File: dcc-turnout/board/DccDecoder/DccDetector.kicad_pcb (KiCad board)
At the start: 2 copper layers, 60 x 52 mm, 45 parts, among them J1 Conn_01x02, J2 Conn_01x02, J3 Conn_01x03, J4 Conn_01x02, J5 Conn_01x02, J6 Conn_01x02, J7 Conn_01x04, Q1 BC560, Q2 BC807, Q3 BC817, Q4 NXV90EPR, U1 AMS1117-5.0, U2 6N137S1, U3 PC817, U4 AMS1117-3.3

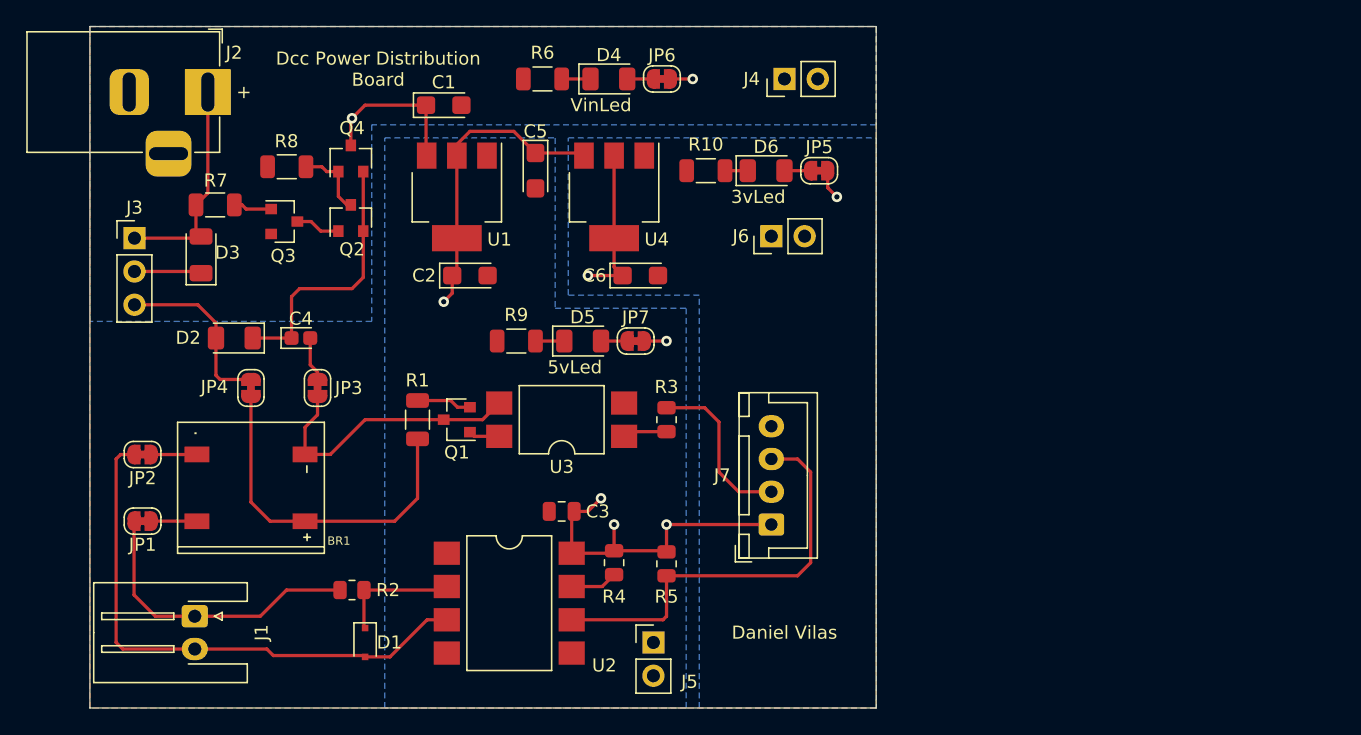
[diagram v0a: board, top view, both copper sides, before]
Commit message: Buck Design
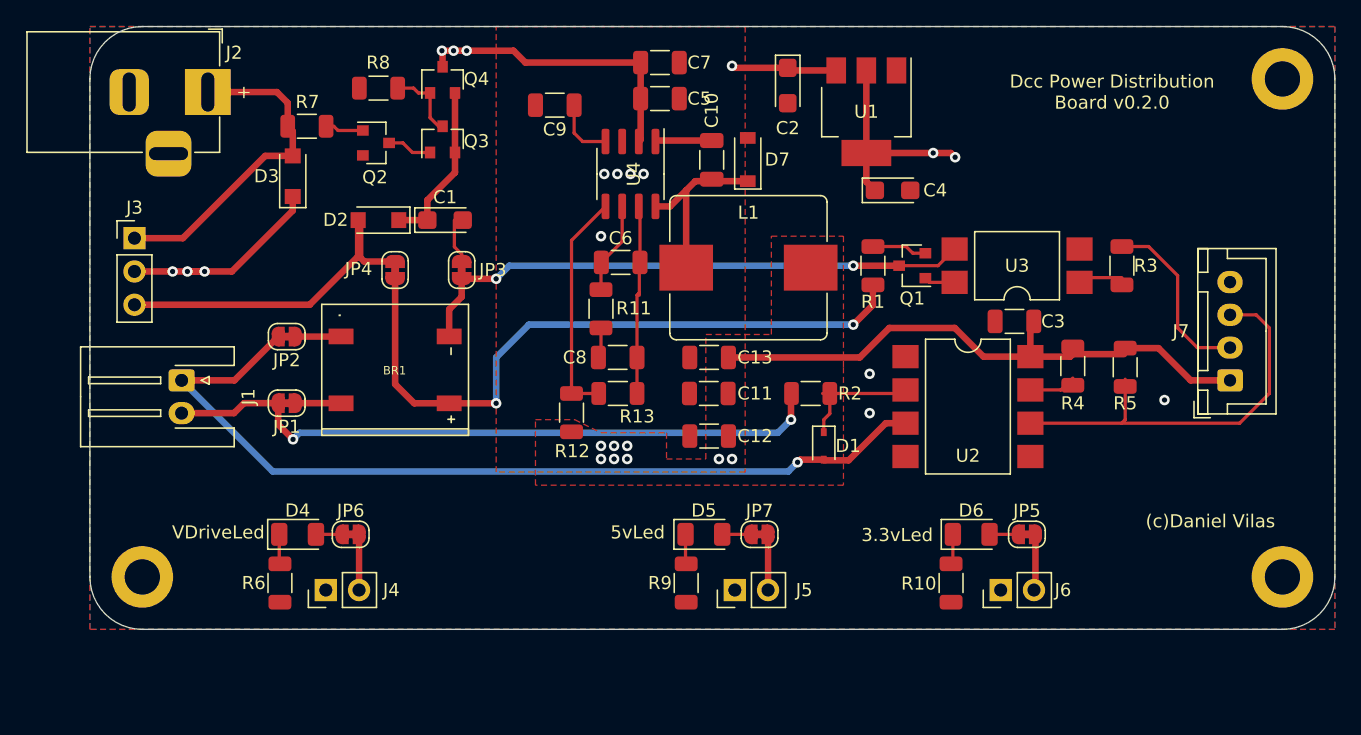
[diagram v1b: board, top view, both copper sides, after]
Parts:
- removed the C1 at (47.0, 26.0)
- removed the C2 at (49.0, 39.0)
- removed the U1 at (48.0, 33.0)
- added C10: 100nf 1m, Capacitor_SMD:C_1206_3216Metric, F.Cu at (67.5, 30.2)
- added C11: 10uf 2m, Capacitor_SMD:C_1206_3216Metric, F.Cu at (67.2, 48.0)
- added C12: 10uf 2m, Capacitor_SMD:C_1206_3216Metric, F.Cu at (67.2, 51.2)
- added C13: 10uf 2m, Capacitor_SMD:C_1206_3216Metric, F.Cu at (67.2, 45.2)
- added C5: 10uf 2m, Capacitor_SMD:C_1206_3216Metric, F.Cu at (63.5, 25.5)
- added C6: 10pf, Capacitor_SMD:C_1206_3216Metric, F.Cu at (60.5, 38.0)
- added C7: 10uf 2m, Capacitor_SMD:C_1206_3216Metric, F.Cu at (63.5, 22.8)
- added C8: 5.6nf, Capacitor_SMD:C_1206_3216Metric, F.Cu at (60.3, 45.2)
- added C9: 8.2nf, Capacitor_SMD:C_1206_3216Metric, F.Cu at (55.5, 26.0)
- added D7: SS24A+, Diode_SMD:D_SOD-123, F.Cu at (70.2, 30.1)
- added H1: MountingHole_Pad, MountingHole:MountingHole_2.7mm_M2.5_DIN965_Pad, F.Cu at (24.0, 62.0)
- added H2: MountingHole_Pad, MountingHole:MountingHole_2.7mm_M2.5_DIN965_Pad, F.Cu at (111.0, 62.0)
- added H3: MountingHole_Pad, MountingHole:MountingHole_2.7mm_M2.5_DIN965_Pad, F.Cu at (111.0, 24.0)
- added L1: 22uH 75mO, Project:L_Bourns_SRP1035, F.Cu at (70.2, 38.4)
- added R11: 5.62K, Resistor_SMD:R_1206_3216Metric, F.Cu at (59.0, 41.5)
- added R12: 10.2K, Resistor_SMD:R_1206_3216Metric, F.Cu at (56.8, 49.5)
- added R13: 1.96K, Resistor_SMD:R_1206_3216Metric, F.Cu at (60.3, 48.0)
- added U4: TPS54331D, Package_SO:SOIC-8_3.9x4.9mm_P1.27mm, F.Cu at (61.2, 31.2)
- C1: renamed from C4; value 10u -> 10uf; footprint Capacitor_Tantalum_SMD:CP_EIA-1608-08_AVX-J -> Capacitor_Tantalum_SMD:CP_EIA-3216-18_Kemet-A
- C3: footprint Capacitor_SMD:C_0805_2012Metric -> Capacitor_SMD:C_1206_3216Metric
- D1: footprint Diode_SMD:D_SOD-323F -> Diode_SMD:D_SOD-323
- D2, D3: value D -> GS1510FL; footprint Diode_SMD:D_1206_3216Metric -> Project:D_SOD-123FL
- Q1: value BC560 -> BC857
- Q4: value NXV90EPR -> BSS308
- R2, R3, R4, R5: footprint Resistor_SMD:R_0805_2012Metric -> Resistor_SMD:R_1206_3216Metric
- R8: value 100k -> 100K
- moved J4 52.4 mm to (38.0, 63.0)
- moved R6 43.4 mm to (34.5, 62.5), turned to 270 degrees
- moved D4 42.1 mm to (35.9, 58.8)
- moved JP6 42.1 mm to (39.9, 58.8)
- moved D1 38.1 mm to (76.0, 52.0)
- moved R2 38.1 mm to (75.0, 48.0)
- moved R4 38.1 mm to (95.0, 45.9)
- moved R5 38.1 mm to (99.0, 46.0)
- moved U2 38.1 mm to (87.0, 49.0)
- moved C3 37.5 mm to (90.5, 42.5)
- moved J7 36.7 mm to (107.0, 47.0)
- moved Q1 36.7 mm to (82.8, 38.2)
- moved R1 36.7 mm to (79.8, 38.2)
- moved R3 36.7 mm to (98.8, 38.2)
- moved U3 36.7 mm to (90.8, 38.2)
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- renumbered C5 to C2, C6 to C4, Q3 to Q2, Q2 to Q3, U4 to U1
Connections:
- net Net-(BR1-Pad+) renamed /Dcc Interface/DccP+
- net Net-(BR1-Pad-) renamed /Dcc Interface/DccP-
- net Net-(C4-Pad1) renamed /Power Distribution/_DccVinP
- J1 pad 1: /Dcc Interface/J -> /Dcc Interface/K
- J1 pad 2: /Dcc Interface/K -> /Dcc Interface/J
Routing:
- net /Dcc Interface/J: track 22.9 -> 51.5 mm, vias 0 -> 2
- net /Dcc Interface/K: track 42.4 -> 68.4 mm, vias 0 -> 1
- net /Dcc Interface/DccP+: track 26.6 -> 51.8 mm, vias 0 -> 2
- net Vdrive: track 18.9 -> 43.1 mm, vias 2 -> 6
- net /Dcc Interface/DccP-: track 21.3 -> 43.4 mm, vias 0 -> 2
- net Net-(R12-Pad2): track 0.00 -> 17.4 mm
- net GND: track 3.39 -> 18.0 mm, vias 0 -> 8
- net /Power Distribution/_PH: track 0.00 -> 13.7 mm
- net /Dcc Interface/DccPower: track 13.6 -> 27.0 mm
- net /Power Distribution/Vin: track 16.7 -> 25.3 mm
- net /Power Distribution/_DccVinP: track 20.3 -> 12.8 mm
- net Net-(C6-Pad1): track 0.00 -> 7.02 mm
- net +5V: track 50.2 -> 56.7 mm, vias 5 -> 9
- net +3V3: track 14.4 -> 20.8 mm
- net Net-(C9-Pad1): track 0.00 -> 4.79 mm
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- added copper zone on In2.Cu, net +3V3
- added copper zone on F.Cu, net +5V
- added copper zone on In2.Cu, net +5V
- added copper zone on B.Cu, net GND
- added copper zone on In1.Cu, net GND
- added copper zone on In2.Cu, net Vdrive
- removed copper zone on B.Cu, net +3V3
- removed copper zone on B.Cu, net +5V
- removed copper zone on B.Cu, net Vdrive
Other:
- board size 60 x 52 mm -> 95 x 46 mm
- copper layers 2 -> 4
- net class Power added: clearance 0.3, trace_width 0.5, via_dia 0.8, via_drill 0.4
- board text added: "(c)Daniel Vilas"
- board text added: "+ 5V -"
- board text added: "3.3vLed"
- board text added: "Dcc Power Distribution Board v0.2.0"
- board text added: "VDriveLed"
- board text removed: "3vLed"
- board text removed: "Daniel Vilas"
- board text removed: "GND 5V"
- board text removed: "VinLed"
